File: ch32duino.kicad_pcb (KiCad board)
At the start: 2 copper layers, 48.3 x 17.8 mm, 6 parts, among them J1 Analog, J2 Digital

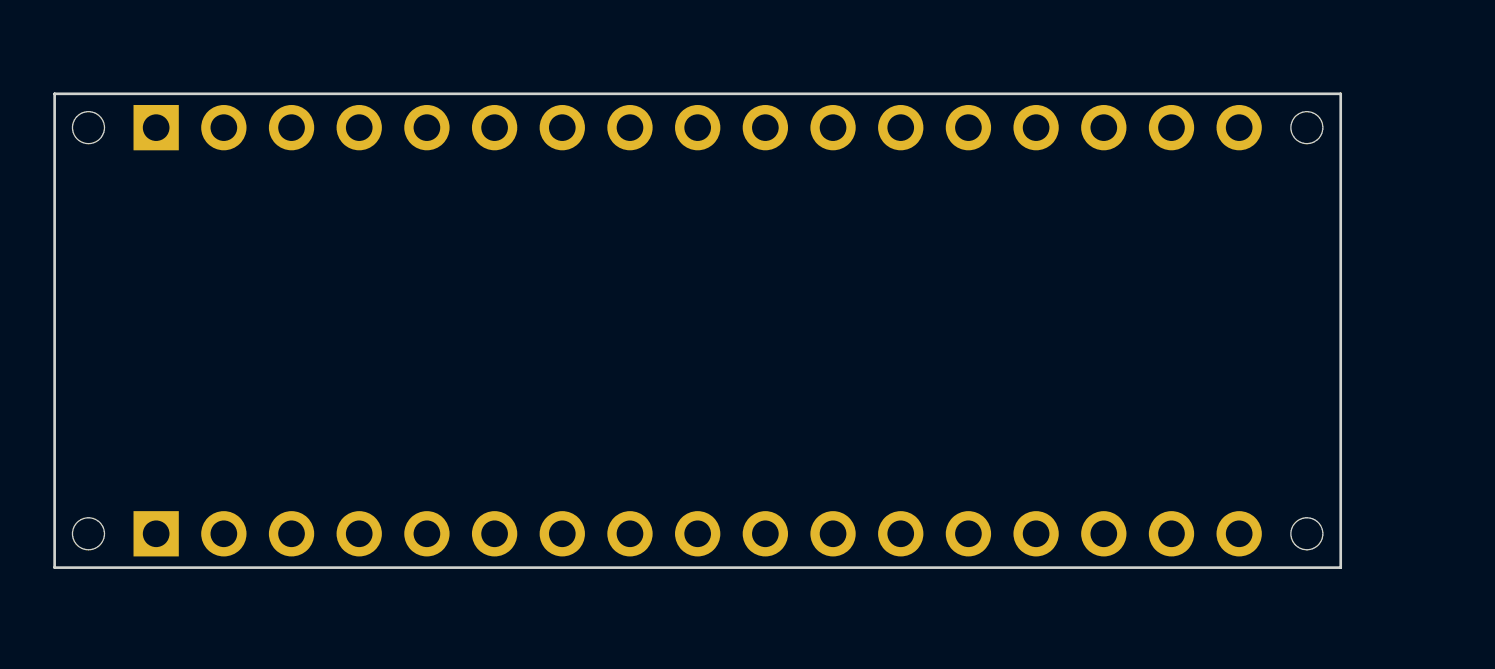
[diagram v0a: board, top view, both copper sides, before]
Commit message: do layout and routing
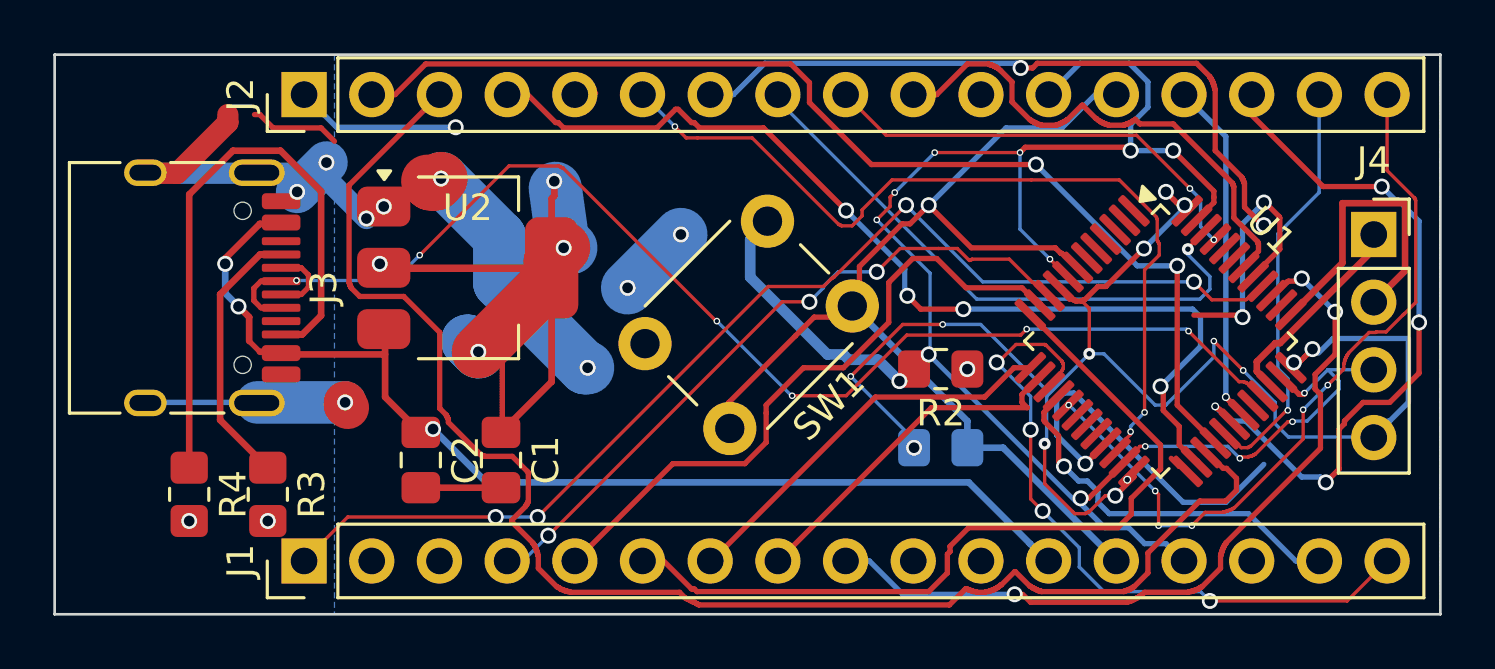
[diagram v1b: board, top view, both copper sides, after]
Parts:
- removed MH1, MH2, MH3, MH4: MountingHole_1.2mm, Arduino_MountingHole:MountingHole_1.2mm
- added C1: 100nF, Capacitor_SMD:C_0805_2012Metric_Pad1.18x1.45mm_HandSolder, F.Cu at (116.8, 96.0)
- added C2: 100nF, Capacitor_SMD:C_0805_2012Metric_Pad1.18x1.45mm_HandSolder, F.Cu at (113.7, 96.0)
- added J3: USB_C_Receptacle_USB2.0_14P, Connector_USB:USB_C_Receptacle_HRO_TYPE-C-31-M-12, F.Cu at (104.5, 89.5)
- added J4: ICSP, Connector_PinSocket_2.54mm:PinSocket_1x04_P2.54mm_Vertical, F.Cu at (149.5, 87.5)
- added R1: 10k, Resistor_SMD:R_0805_2012Metric_Pad1.20x1.40mm_HandSolder, B.Cu at (133.2, 95.5)
- added R2: 10k, Resistor_SMD:R_0805_2012Metric_Pad1.20x1.40mm_HandSolder, F.Cu at (133.2, 92.5)
- added R3: 5.1k, Resistor_SMD:R_0805_2012Metric_Pad1.20x1.40mm_HandSolder, F.Cu at (108.0, 97.2)
- added R4: 5.1k, Resistor_SMD:R_0805_2012Metric_Pad1.20x1.40mm_HandSolder, F.Cu at (105.0, 97.2)
- added SW1: SW_Push, Button_Switch_THT:SW_PUSH_6mm, F.Cu at (129.9, 90.2)
- added U1: CH32V203CxTx, Package_QFP:LQFP-48_7x7mm_P0.5mm, F.Cu at (141.5, 91.5)
- added U2: AMS1117-3.3, Package_TO_SOT_SMD:SOT-223-3_TabPin2, F.Cu at (115.5, 88.8)
- J1, J2: moved to F.Cu
- moved J2 5.69 mm to (109.4, 82.2), turned to 90 degrees
- moved J1 5.64 mm to (109.4, 99.8), turned to 90 degrees
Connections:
- J1 pad 15: VCC -> +3V3
- J1 pad 3: /AREF -> +3V3
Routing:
- net GND: track 0.00 -> 117.6 mm, vias 0 -> 25
- net +3V3: track 0.00 -> 95.5 mm, vias 0 -> 18
- net /*D10: track 0.00 -> 56.0 mm
- net /USB D+: track 0.00 -> 46.3 mm, vias 0 -> 6
- net /*D13: track 0.00 -> 42.5 mm, vias 0 -> 4
- net +5V: track 0.00 -> 41.6 mm, vias 0 -> 3
- net /*D11: track 0.00 -> 41.5 mm, vias 0 -> 2
- net /~{RESET}: track 0.00 -> 40.9 mm, vias 0 -> 1
- net /*D6: track 0.00 -> 40.1 mm, vias 0 -> 3
- net /*D9: track 0.00 -> 36.9 mm, vias 0 -> 4
- net /D7: track 0.00 -> 32.3 mm, vias 0 -> 3
- net /A2: track 0.00 -> 30.3 mm
- net /A5: track 0.00 -> 29.5 mm, vias 0 -> 3
- net /D16/MOSI: track 0.00 -> 28.2 mm, vias 0 -> 6
- net /D1/TX: track 0.00 -> 26.7 mm, vias 0 -> 4
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- added copper zone on B.Cu, net +3V3
- added copper zone on F.Cu, net GND
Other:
- board size 48.3 x 17.8 mm -> 52 x 21 mm
- board text removed: "ICSP"
- board text removed: "USB Micro-B"
